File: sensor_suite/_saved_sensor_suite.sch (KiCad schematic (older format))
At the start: 28 parts, among them CN1 609-3634-ND, J1 Bar02, J2 Conn_02x10_Counter_Clockwise, J3 Conn_01x02, J4 Conn_01x02, J5 LSM303, J6 Conn_02x20_Counter_Clockwise, J7 Conn_01x03_Female, J8 Conn_01x10, U1 MAX6581, U2 Pi3+, U3 LM3480-3.3

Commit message: Swapped out Gyro
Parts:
- removed J5: LSM303, Connector_PinHeader_2.54mm:PinHeader_1x08_P2.54mm_Vertical, symbol Connector_Generic:Conn_01x08
- added C11: C_Small, Capacitor_SMD:C_0805_2012Metric_Pad1.15x1.40mm_HandSolder, symbol Device:C_Small
- added J5: Conn_01x04_Female, Connector_PinHeader_2.54mm:PinHeader_1x04_P2.54mm_Vertical, symbol Connector:Conn_01x04_Female
- U2: footprint ROV:Pi3+ -> rov:Pi3+; symbol rov:Pi3+ -> _saved_sensor_suite-rescue:Pi3+-rov
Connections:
- wire segments 142 -> 139
- no-connect marks 44 -> 41
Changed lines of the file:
@@
 	8750 1950 8750 5400
-$Comp
-L Connector_Generic:Conn_01x08 J5
-U 1 1 5C1E8E53
-P 6800 4000
-F 0 "J5" H 6879 3992 50  0000 L CNN
-F 1 "LSM303" H 6879 3901 50  0000 L CNN
-F 2 "Connector_PinHeader_2.54mm:PinHeader_1x08_P2.54mm_Vertical" H 6800 4000 50  0001 C CNN
-F 3 "~" H 6800 4000 50  0001 C CNN
-	1    6800 4000
-	1    0    0    -1
-$EndComp
 $Comp
 L Connector_Generic:Conn_01x04 J1
@@
 $EndComp
 Wire Wire Line
-	6600 4200 6400 4200
-Wire Wire Line
-	6400 4200 6400 4250
-$Comp
-L power:+3.3V #PWR0105
-U 1 1 5C1E8E55
-P 7300 4250
-F 0 "#PWR0105" H 7300 4100 50  0001 C CNN
-F 1 "+3.3V" H 7315 4423 50  0000 C CNN
-F 2 "" H 7300 4250 50  0001 C CNN
-F 3 "" H 7300 4250 50  0001 C CNN
-	1    7300 4250
-	1    0    0    -1
-$EndComp
-Wire Wire Line
-	7300 4400 7300 4300
-Wire Wire Line
-	6600 4400 7300 4400
-Wire Wire Line
-	6600 4300 7300 4300
-Connection ~ 7300 4300
-Wire Wire Line
-	7300 4300 7300 4250
-Wire Wire Line
-	6600 3900 6400 3900
-Wire Wire Line
-	6600 4000 6400 4000
-Wire Wire Line
-	6600 4100 6400 4100
-Wire Wire Line
-	6600 3800 6400 3800
-Wire Wire Line
-	6600 3700 6400 3700
-Wire Wire Line
 	1250 1800 1200 1800
 Wire Wire Line
@@
 Wire Wire Line
 	3400 5250 3200 5250
-NoConn ~ 6400 3900
-NoConn ~ 6400 4000
-NoConn ~ 6400 4100
 $Comp
 L power:GNDS #PWR0107
@@
 Text GLabel 9700 1750 0    50   Input ~ 0
 SCL_iso
-Text GLabel 6400 3700 0    50   Input ~ 0
-SDA_iso
-Text GLabel 6400 3800 0    50   Input ~ 0
-SCL_iso
 Text GLabel 3700 4950 0    50   Input ~ 0
 SDA_iso
@@
 $EndComp
 $Comp
-L rov:Pi3+ U2
+L _saved_sensor_suite-rescue:Pi3+-rov U2
 U 1 1 5C47740E
 P 2950 3800
 F 0 "U2" H 3128 3846 50  0000 L CNN
 F 1 "Pi3+" H 3128 3755 50  0000 L CNN
-F 2 "ROV:Pi3+" H 2950 3800 50  0001 C CNN
+F 2 "rov:Pi3+" H 2950 3800 50  0001 C CNN
 F 3 "" H 2950 3800 50  0001 C CNN
 	1    2950 3800
@@
 $EndComp
 $Comp
-L power:GNDPWR #PWR0104
-U 1 1 5C6D8CD0
-P 6400 4250
-F 0 "#PWR0104" H 6400 4050 50  0001 C CNN
-F 1 "GNDPWR" H 6404 4096 50  0000 C CNN
-F 2 "" H 6400 4200 50  0001 C CNN
-F 3 "" H 6400 4200 50  0001 C CNN
-	1    6400 4250
-	1    0    0    -1
-$EndComp
-$Comp
 L power:GNDPWR #PWR0106
 U 1 1 5C6D9A43
@@
 NoConn ~ 2300 5250
 NoConn ~ 2300 5750
+$Comp
+L Connector:Conn_01x04_Female J5
+U 1 1 5C7E2578
+P 7150 3750
+F 0 "J5" H 7177 3726 50  0000 L CNN
+F 1 "Conn_01x04_Female" H 7177 3635 50  0000 L CNN
+F 2 "Connector_PinHeader_2.54mm:PinHeader_1x04_P2.54mm_Vertical" H 7150 3750 50  0001 C CNN
+F 3 "~" H 7150 3750 50  0001 C CNN
+	1    7150 3750
+	1    0    0    -1
+$EndComp
+$Comp
+L Device:C_Small C11
+U 1 1 5C7EC20F
+P 6450 3800
+F 0 "C11" H 6250 3850 50  0000 L CNN
+F 1 "C_Small" H 6050 3750 50  0000 L CNN
+F 2 "Capacitor_SMD:C_0805_2012Metric_Pad1.15x1.40mm_HandSolder" H 6450 3800 50  0001 C CNN
+F 3 "~" H 6450 3800 50  0001 C CNN
+	1    6450 3800
+	1    0    0    -1
+$EndComp
+Text GLabel 6950 3850 0    50   Input ~ 0
+SDA_iso
+Text GLabel 6950 3950 0    50   Input ~ 0
+SCL_iso
+Wire Wire Line
+	6450 3600 6450 3650
+Connection ~ 6450 3650
+Wire Wire Line
+	6450 3650 6450 3700
+Wire Wire Line
+	6450 3900 6450 3950
+Wire Wire Line
+	6450 3650 6950 3650
+Wire Wire Line
+	6950 3750 6550 3750
+Wire Wire Line
+	6550 3750 6550 3950
+Wire Wire Line
+	6550 3950 6450 3950
+Connection ~ 6450 3950
+Wire Wire Line
+	6450 3950 6450 4000
+$Comp
+L power:+3.3V #PWR0104
+U 1 1 5C8203C7
+P 6450 4000
+F 0 "#PWR0104" H 6450 3850 50  0001 C CNN
+F 1 "+3.3V" H 6465 4173 50  0000 C CNN
+F 2 "" H 6450 4000 50  0001 C CNN
+F 3 "" H 6450 4000 50  0001 C CNN
+	1    6450 4000
+	-1   0    0    1
+$EndComp
+$Comp
+L power:GNDPWR #PWR0105
+U 1 1 5C8204EA
+P 6450 3600
+F 0 "#PWR0105" H 6450 3400 50  0001 C CNN
+F 1 "GNDPWR" H 6455 3445 50  0000 C CNN
+F 2 "" H 6450 3550 50  0001 C CNN
+F 3 "" H 6450 3550 50  0001 C CNN
+	1    6450 3600
+	-1   0    0    1
+$EndComp
 $EndSCHEMATC

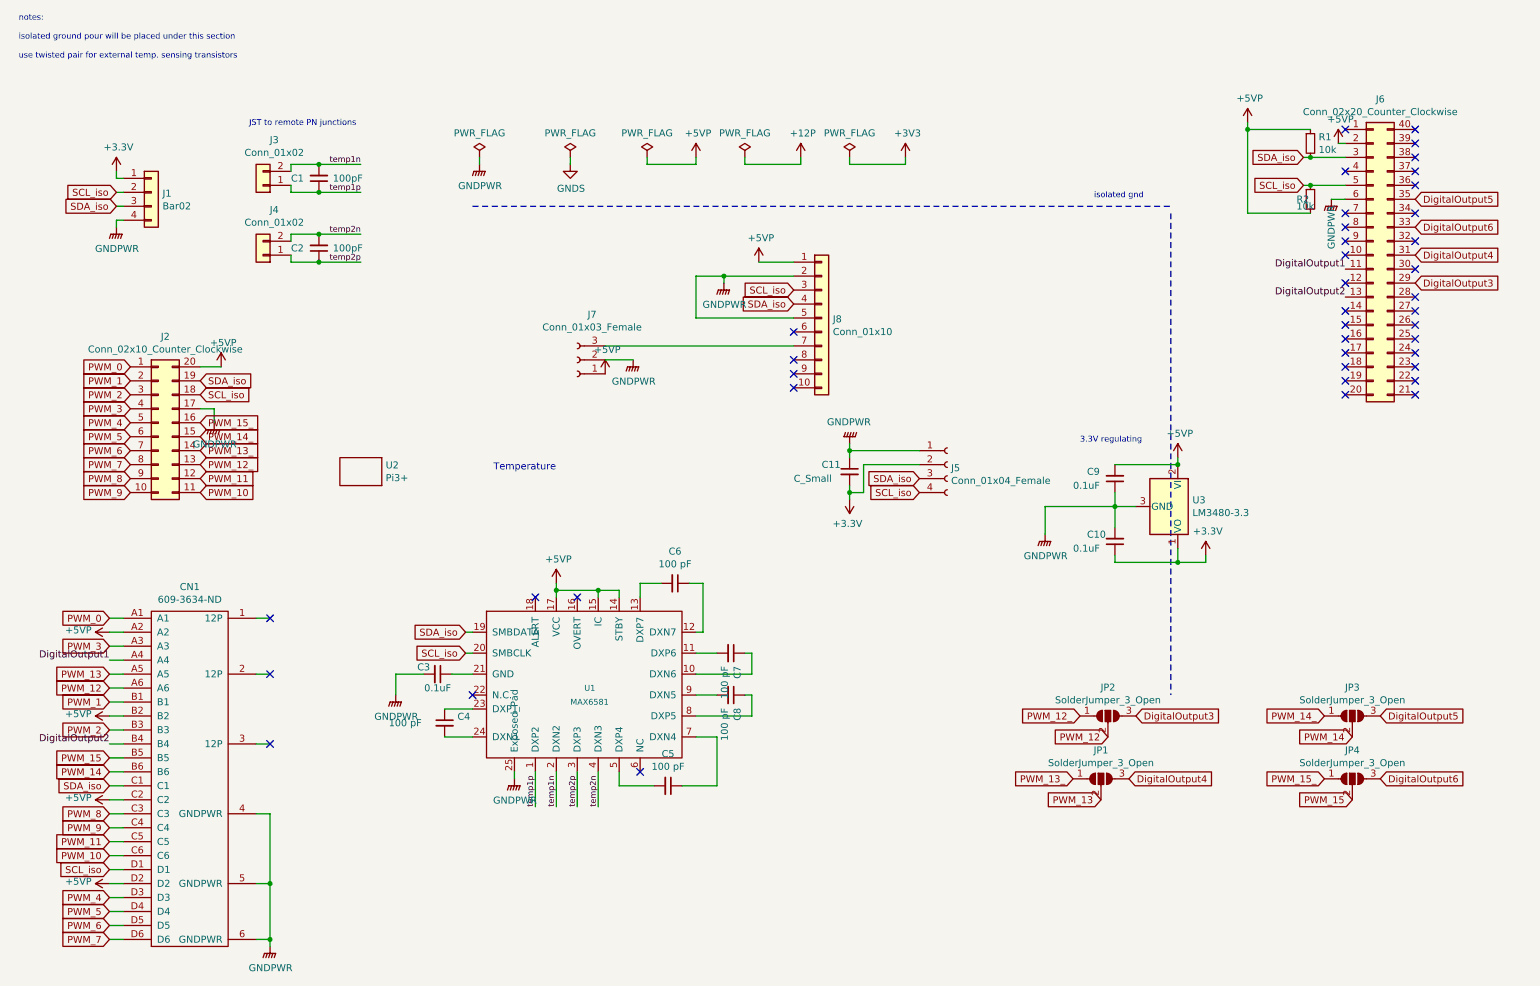
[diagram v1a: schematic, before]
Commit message: sensor board
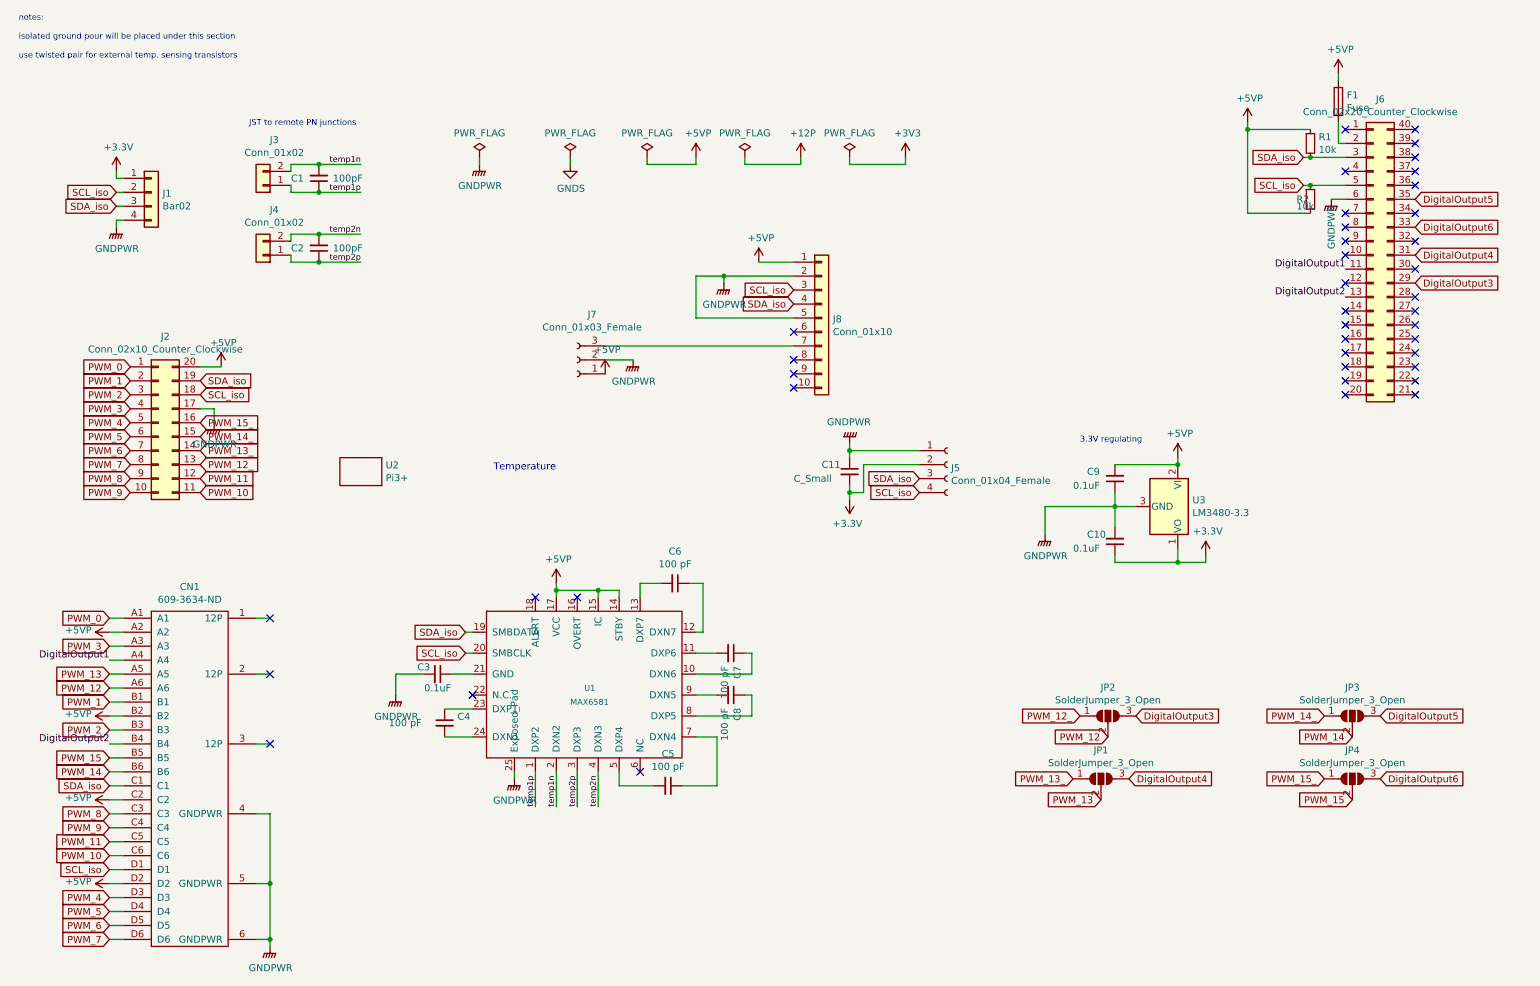
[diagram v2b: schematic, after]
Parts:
- added F1: Fuse, Fuse:Fuse_1812_4532Metric_Pad1.30x3.40mm_HandSolder, symbol Device:Fuse
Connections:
- net +5VP: now also F1.1; no longer J6.2 (Pin_2)
- new net: F1.2, J6.2 (Pin_2)
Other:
- note removed: "isolated gnd\n"
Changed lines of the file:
@@
 Wire Wire Line
 	7850 4050 8350 4050
-Text Notes 8200 1850 0    42   ~ 0
-isolated gnd\n
 Text Label 4350 6200 1    42   ~ 0
 temp1n
@@
 Text Notes 3900 3800 0    50   ~ 0
 Temperature\n
-Wire Notes Line
-	3750 1900 8750 1900
-Wire Notes Line
-	8750 1950 8750 5400
 $Comp
 L Connector_Generic:Conn_01x04 J1
@@
 L power:+5VP #PWR0126
 U 1 1 5C73E075
-P 9950 1450
-F 0 "#PWR0126" H 9950 1300 50  0001 C CNN
-F 1 "+5VP" H 9965 1623 50  0000 C CNN
-F 2 "" H 9950 1450 50  0001 C CNN
-F 3 "" H 9950 1450 50  0001 C CNN
-	1    9950 1450
+P 9950 950
+F 0 "#PWR0126" H 9950 800 50  0001 C CNN
+F 1 "+5VP" H 9965 1123 50  0000 C CNN
+F 2 "" H 9950 950 50  0001 C CNN
+F 3 "" H 9950 950 50  0001 C CNN
+	1    9950 950
 	1    0    0    -1
 $EndComp
@@
 	-1   0    0    1
 $EndComp
+$Comp
+L Device:Fuse F1
+U 1 1 5C80BCEF
+P 9950 1150
+F 0 "F1" H 10010 1196 50  0000 L CNN
+F 1 "Fuse" H 10010 1105 50  0000 L CNN
+F 2 "Fuse:Fuse_1812_4532Metric_Pad1.30x3.40mm_HandSolder" V 9880 1150 50  0001 C CNN
+F 3 "~" H 9950 1150 50  0001 C CNN
+	1    9950 1150
+	1    0    0    -1
+$EndComp
+Wire Wire Line
+	9950 1000 9950 950
+Wire Wire Line
+	9950 1300 9950 1450
 $EndSCHEMATC
